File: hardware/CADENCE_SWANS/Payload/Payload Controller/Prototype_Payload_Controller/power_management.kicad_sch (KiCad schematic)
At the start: 54 parts, among them U3 LT8612, U5 LT8612, U6 LT8612

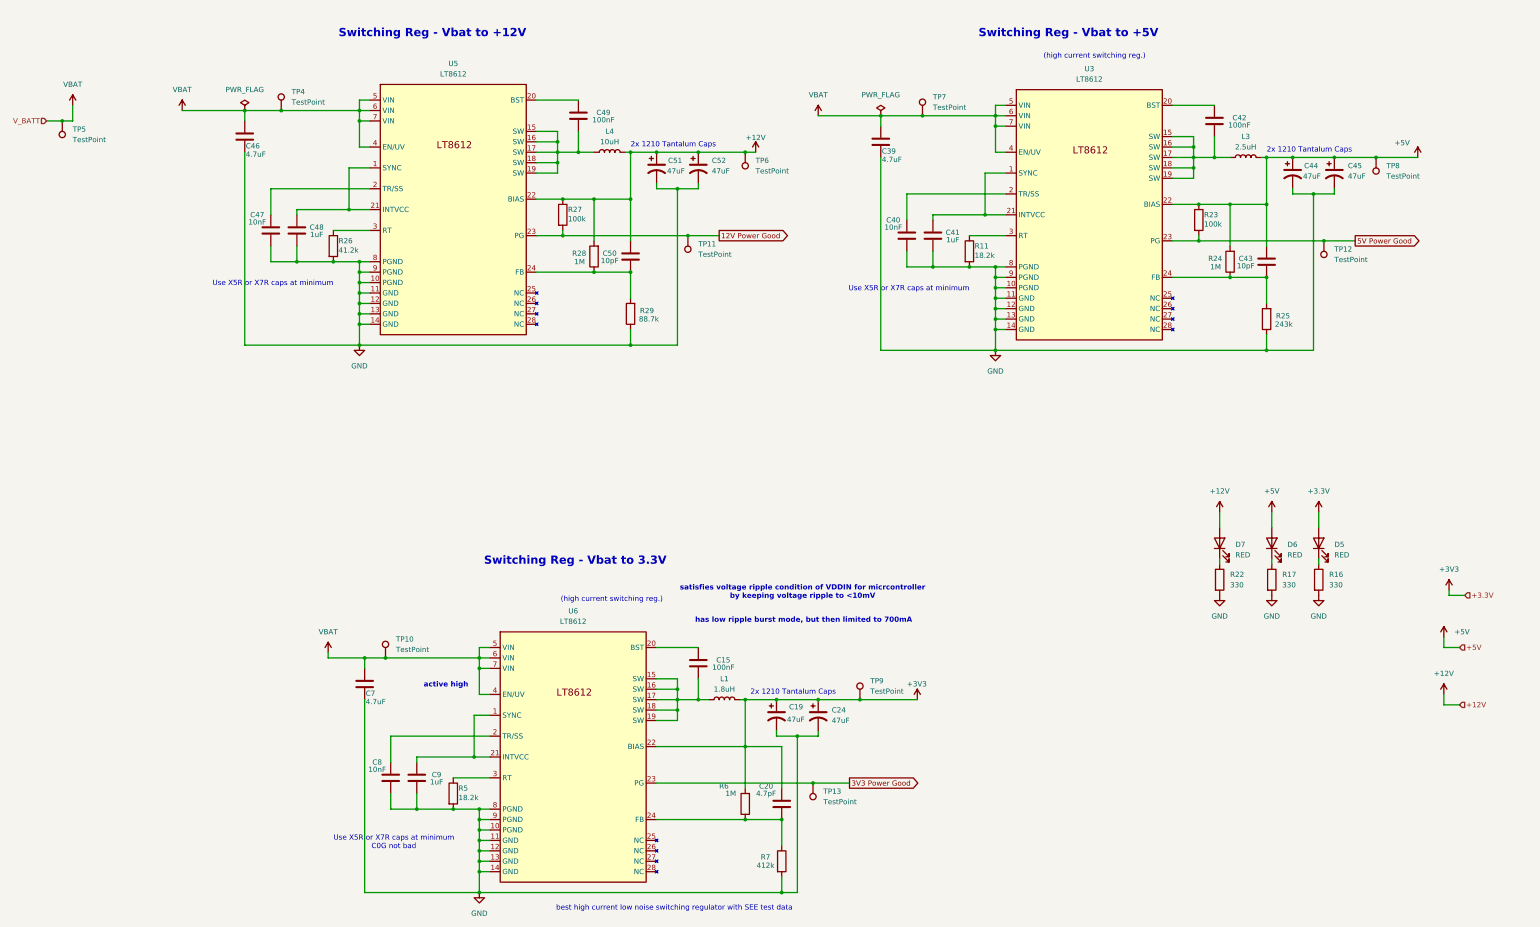
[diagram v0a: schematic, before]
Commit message: updates
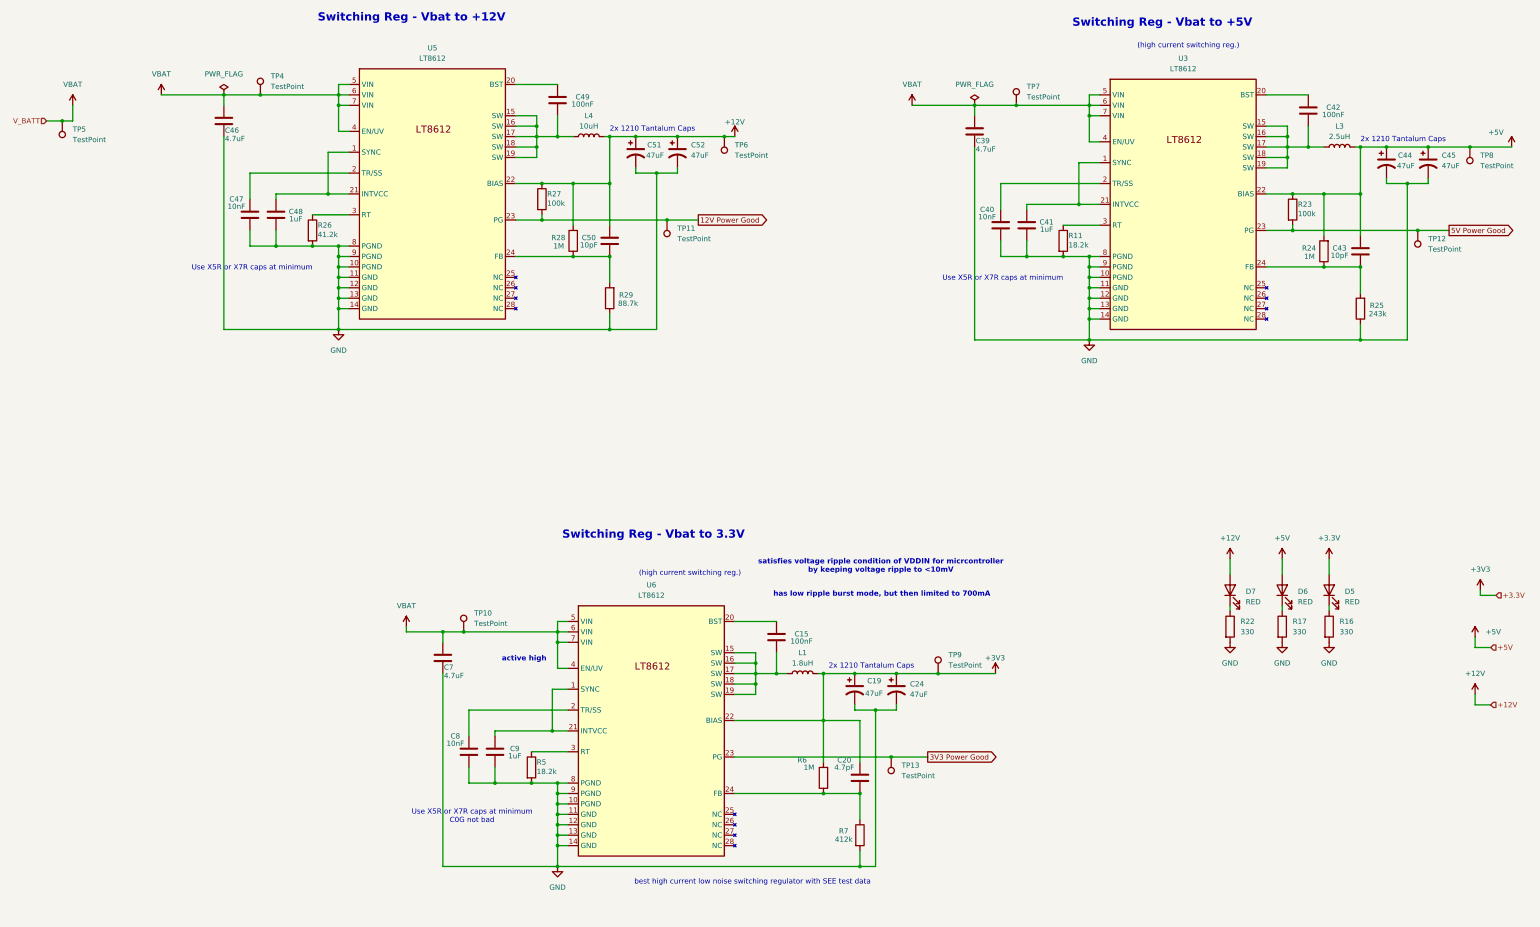
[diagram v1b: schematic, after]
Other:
- moved on the sheet: C15, C19, C20, C24, C39, C40, C41, C42, C43, C44, C45, C46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
